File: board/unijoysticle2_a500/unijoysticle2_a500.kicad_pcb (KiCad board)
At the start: 4 copper layers, 67 x 52 mm, 54 parts, among them J1 USB_B_Micro, J2 PORT JOY #1, J3 PORT JOY #2, Q1 S8050, Q2 S8050, SW1 RESET, SW2 BOOT, SW3 MOUSE, SW4 SWAP, U1 ESP32-WROOM-32E, U2 AMS1117-3.3, U3 CH340C, U4 74HC05, U5 74HC05, U6 74HC05

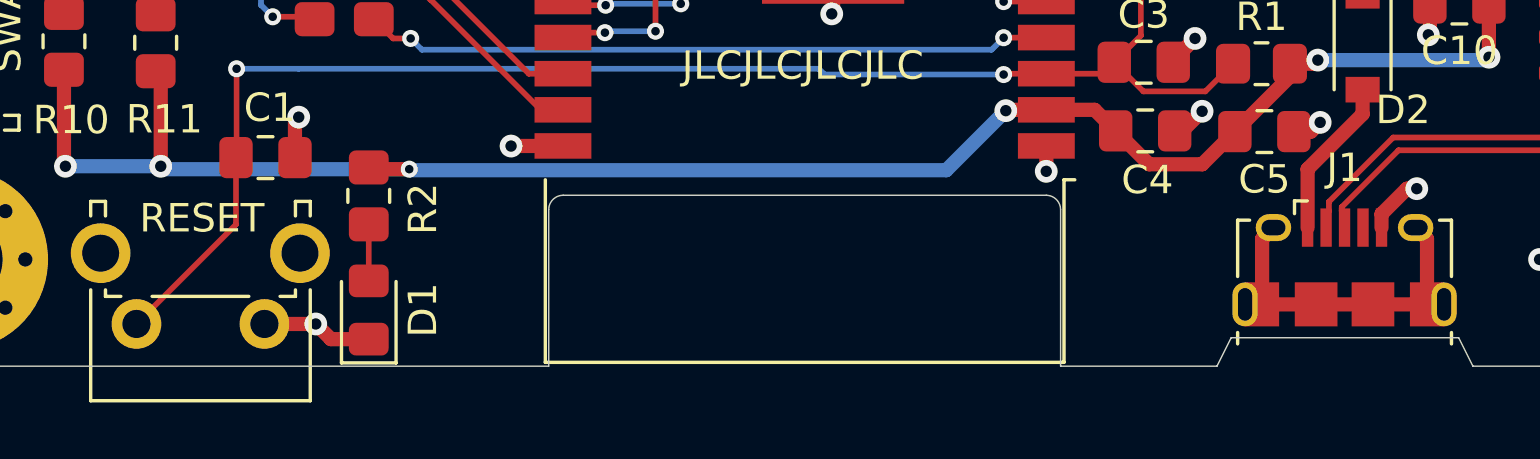
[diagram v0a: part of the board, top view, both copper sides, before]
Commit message: uni a500: add JV
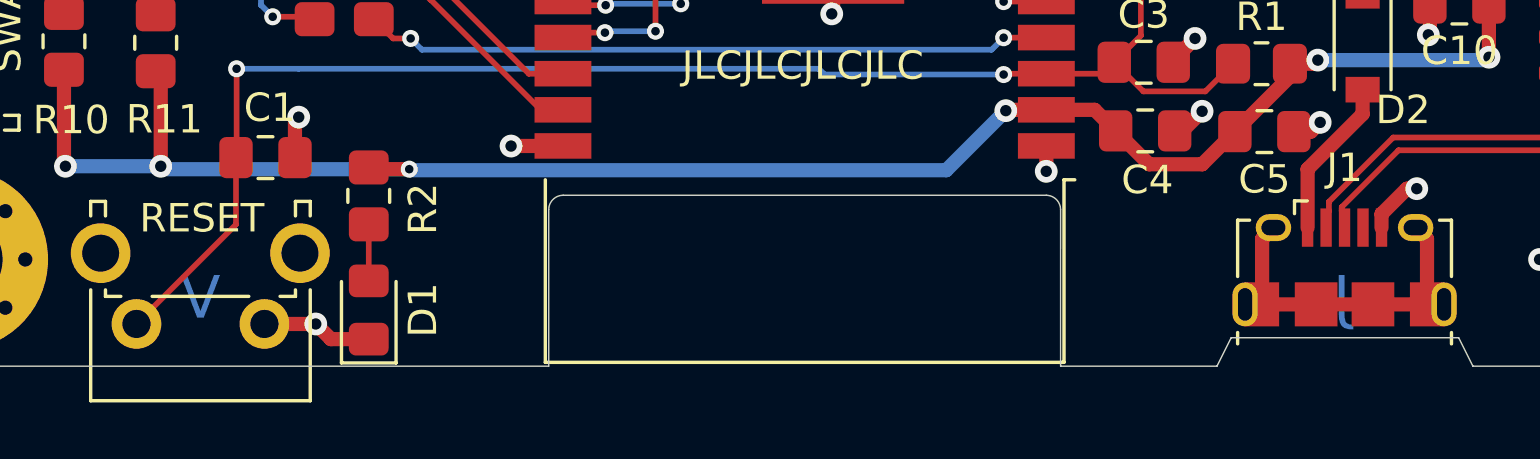
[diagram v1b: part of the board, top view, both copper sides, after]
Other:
- board text added: "J"
- board text added: "V"
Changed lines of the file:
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@@
       (drillshape 0)
       (scaleselection 1)
-      (outputdirectory "gerber_a/")
+      (outputdirectory "assembly_a/")
     )
   )
@@
   (gr_line (start 128.5 147) (end 128 148) (layer "Edge.Cuts") (width 0.05))
   (gr_line (start 121.99259 141.98961) (end 105.00721 141.98961) (layer "Edge.Cuts") (width 0.05))
+  (gr_text "V" (at 92.2528 145.6) (layer "B.Cu")
+    (effects (font (size 1.5 1.5) (thickness 0.3)))
+  )
+  (gr_text "J" (at 132.3848 145.6) (layer "B.Cu")
+    (effects (font (size 1.5 1.5) (thickness 0.3)) (justify mirror))
+  )
   (gr_text "Unijoysticle 2 A500\nRev. A" (at 113.62 131.185) (layer "B.SilkS")
     (effects (font (size 1.5 1.5) (thickness 0.3)) (justify mirror))
